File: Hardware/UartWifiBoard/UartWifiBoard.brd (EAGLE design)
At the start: 50 x 40 mm, 39 parts, among them CN1 B2B-XH, CN2 B4B-XH, CN3 B5B-PH, IC1 ESP-WROOM-02, Q1 RN1302, Q2 RN2302, Q3 TLP2368, Q4 TLP2368, Q5 RN2302, SW1 SKRPACE010, SW2 SKRPACE010, U1 NJM2884U1

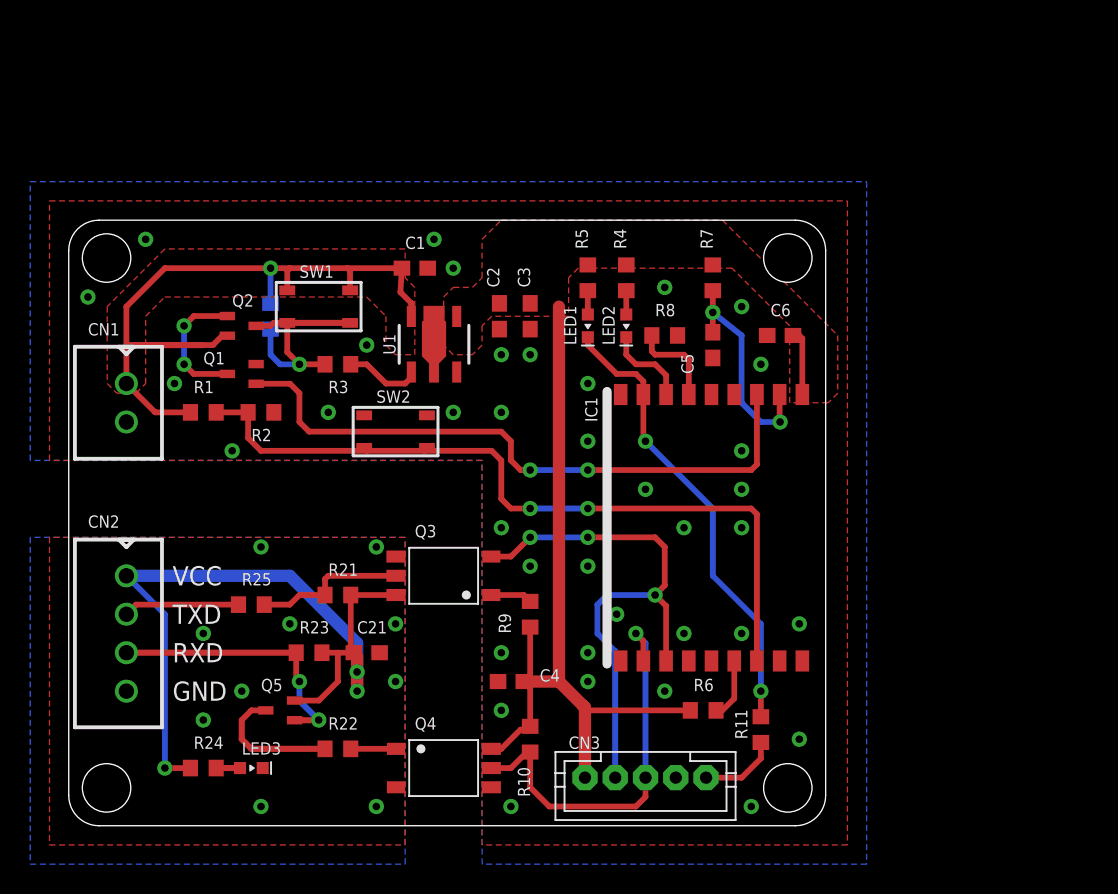
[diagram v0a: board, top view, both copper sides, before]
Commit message: Upload files
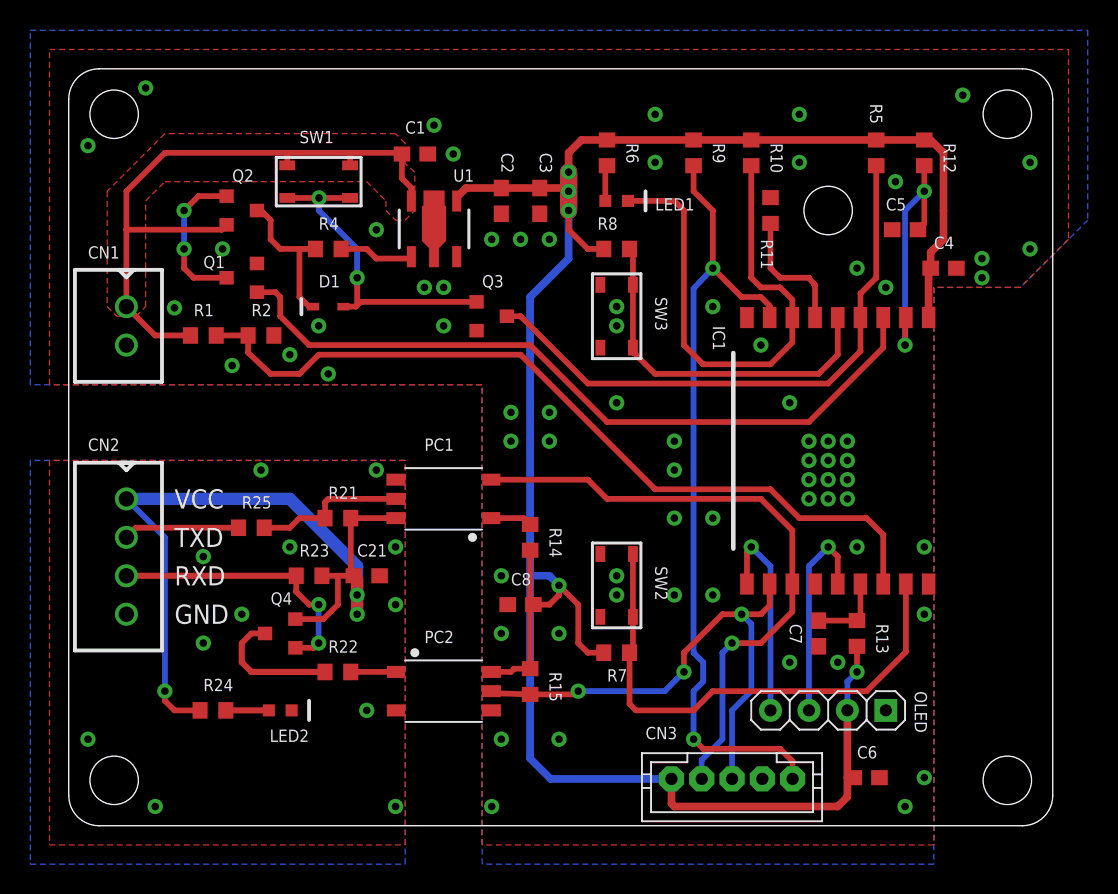
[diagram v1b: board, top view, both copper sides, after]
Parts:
- removed LED3: OSHR1608C1A, optosupply:1608SMD
- removed Q5: RN2302, toshiba:USM
- removed R3: 220, rcl:R0603
- removed R99: 0ohm, rcl:R0603
- added C7, C8: 0.1u, rcl:C0603
- added D1: RB521S30, on-semiconductor:SOD-523F
- added OLED1: DISPLAY-OLED-128X32, generic-brand-oled-modules:DISPLAY-OLED-128X32
- added PC1, PC2: TLP2368, toshiba:SO6-5PIN
- added R12: 10.0k, rcl:R0603
- added R13: 3.3k, rcl:R0603
- added R14: 470, rcl:R0603
- added R15: 1.0k, rcl:R0603
- added SW3: SKRPACE010, alps:SKRP
- C2, C3: value 1.0u -> 2.2u
- LED1: value OSTG1608C1A -> OSOR1608C1A; device optosupply:1608SMD -> optosupply:LED0603SMD
- LED2: value OSYL1608C1A -> OSHR1608C1A; device optosupply:1608SMD -> optosupply:LED0603SMD
- Q1: value RN1302 -> MMUN2211LT1G; device toshiba:USM -> on-semiconductor:SOT-23
- Q2: value RN2302 -> MMUN2111LT1G; device toshiba:USM -> on-semiconductor:SOT-23
- Q3: value TLP2368 -> MMUN2211LT1G; device toshiba:SO6-5PIN -> on-semiconductor:SOT-23
- Q4: value TLP2368 -> MMUN2111LT1G; device toshiba:SO6-5PIN -> on-semiconductor:SOT-23
- R10: value 1.0k -> 3.3k
- R11: value 220 -> 3.3k
- R24: value 3.3k -> 4.7k
- R4: value 3.3k -> 220
- R7, R8: value 10.0k -> 3.3k
- R9: value 470 -> 3.3k
- moved R10 41.4 mm to (45.1, 44.5)
- moved C4 39.5 mm to (57.8, 36.8), turned to 0 degrees
- moved R6 37.4 mm to (35.6, 44.5), turned to 90 degrees
- moved R11 34.3 mm to (46.4, 40.6)
- moved LED2 34.2 mm to (14.0, 7.62), turned to 0 degrees
- moved R9 32.3 mm to (41.3, 44.5), turned to 90 degrees
- moved C6 29.8 mm to (52.7, 3.17), turned to 0 degrees
- moved R7 25.6 mm to (36.2, 11.4), turned to 180 degrees
- moved R5 20.8 mm to (53.3, 44.5)
- moved R4 19.8 mm to (17.1, 38.1), turned to 0 degrees
- moved SW2 17.8 mm to (36.2, 15.9), turned to 270 degrees
- moved Q3 17.4 mm to (27.9, 33.7), turned to 270 degrees
- moved IC1 16.1 mm to (50.8, 24.8)
- moved C5 14.8 mm to (55.2, 39.4), turned to 180 degrees
- moved Q4 14.0 mm to (14.0, 12.7), turned to 90 degrees
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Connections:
- removed net N$10: CN3.5, R11.2
- removed net N$18: IC1.6, R8.2
- removed net N$9: LED2.A, R4.1
- new net IO12: IC1.4, Q3.P$3, R5.1
- new net IO13: IC1.5, R8.1, SW3.1, SW3.2
- new net IO15: IC1.6, R11.2
- new net IO16: IC1.17, R7.1, SW2.1, SW2.2
- new net IO4: IC1.10, OLED1.4
- new net IO5: IC1.14, OLED1.3
- new net N$14: D1.A, Q3.P$1, SW1.3, SW1.4
- net IO0: now also CN3.5, R9.1; no longer LED1.K, R11.1
- net IO2: now also LED1.C, R10.1; no longer LED2.K
- net N$11: now also PC1.5; no longer Q3.5
- net N$13: now also LED2.A; no longer LED3.A
- net N$16: now also PC1.1, R14.1; no longer Q3.1, R9.1
- net N$19: now also R12.1; no longer R7.1
- net N$2: now also R4.2; no longer R3.2
- net N$22: now also R6.1; no longer R5.1
- net N$3: no longer R99.1
- net N$4: now also Q4.P$3; no longer Q5.P$3
- net N$5: now also D1.C, R4.1; no longer R3.1, R99.2, SW1.3, SW1.4
- net N$7: now also Q4.P$1; no longer Q5.P$1
- net N$8: now also PC2.1; no longer Q4.1
- net P+3V3: now also C8.1, OLED1.2, PC2.6, R12.2, R13.2, R14.2, R15.2, R8.2; no longer Q4.6, R4.2
- net PGND: now also C7.2, C8.2, OLED1.1, PC2.4, Q3.P$2, R11.1, SW3.3, SW3.4; no longer Q4.4, R8.1
- net RST: now also C7.1, R13.1; no longer R6.1
- net RXD: now also PC2.5, R15.1; no longer Q4.5, R10.1
- net S+SUP: now also PC1.6, Q4.P$2; no longer Q3.6, Q5.P$2
- net SGND: now also LED2.C, PC1.4, PC2.3; no longer LED3.K, Q3.4, Q4.3
- net TOUT: no longer SW2.1, SW2.2
- net TXD: now also PC1.3; no longer Q3.3
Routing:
- net P+3V3: track 55.9 -> 149.5 mm, vias 0 -> 5
- net IO12: track 0.00 -> 38.8 mm
- net IO16: track 0.00 -> 34.5 mm
- net IO2: track 5.62 -> 34.7 mm
- net IO13: track 0.00 -> 24.0 mm
- net IO0: track 30.5 -> 53.3 mm
- net N$14: track 0.00 -> 21.2 mm, vias 0 -> 2
- net IO5: track 0.00 -> 14.0 mm, vias 0 -> 1
- net IO4: track 0.00 -> 13.9 mm, vias 0 -> 1
- net IO15: track 0.00 -> 8.54 mm
- net RXD: track 26.8 -> 34.7 mm, vias 1 -> 3
- net IO14: track 42.1 -> 49.7 mm, vias 2 -> 0
- net N$18: track 6.03 -> 0.00 mm
- net N$10: track 5.20 -> 0.00 mm
- net TXD: track 36.3 -> 41.3 mm, vias 3 -> 1
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- removed copper zone on layer 1, net P+3V3
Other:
- board size 50 x 40 mm -> 65 x 50 mm
- board text added: "OLED"
- board text added: "SCL"
- board text added: "SDA"
- board text added: "UWB+OLED-04"
- board text removed: "UWB-02"
